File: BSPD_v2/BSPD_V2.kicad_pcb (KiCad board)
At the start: 2 copper layers, 85.5 x 52 mm, 0 parts

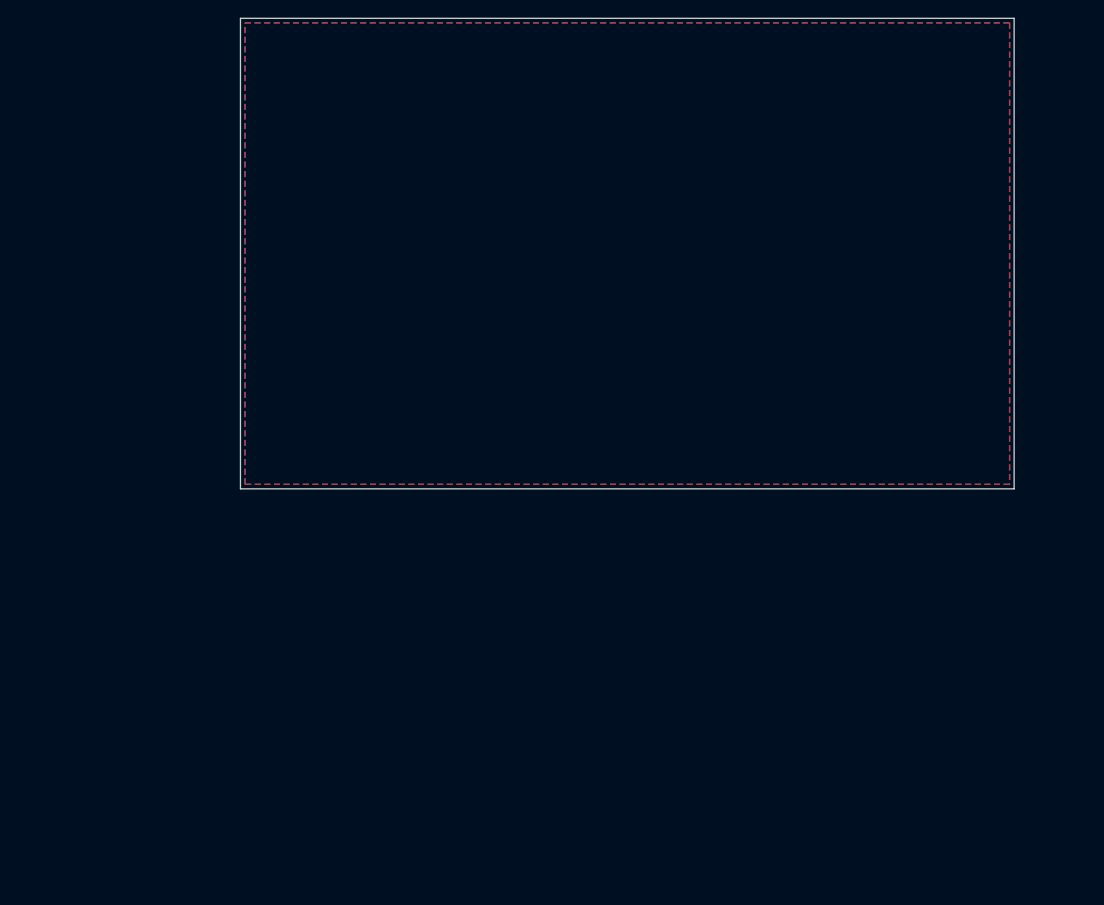
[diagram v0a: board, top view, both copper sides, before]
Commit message: Updated pcb design
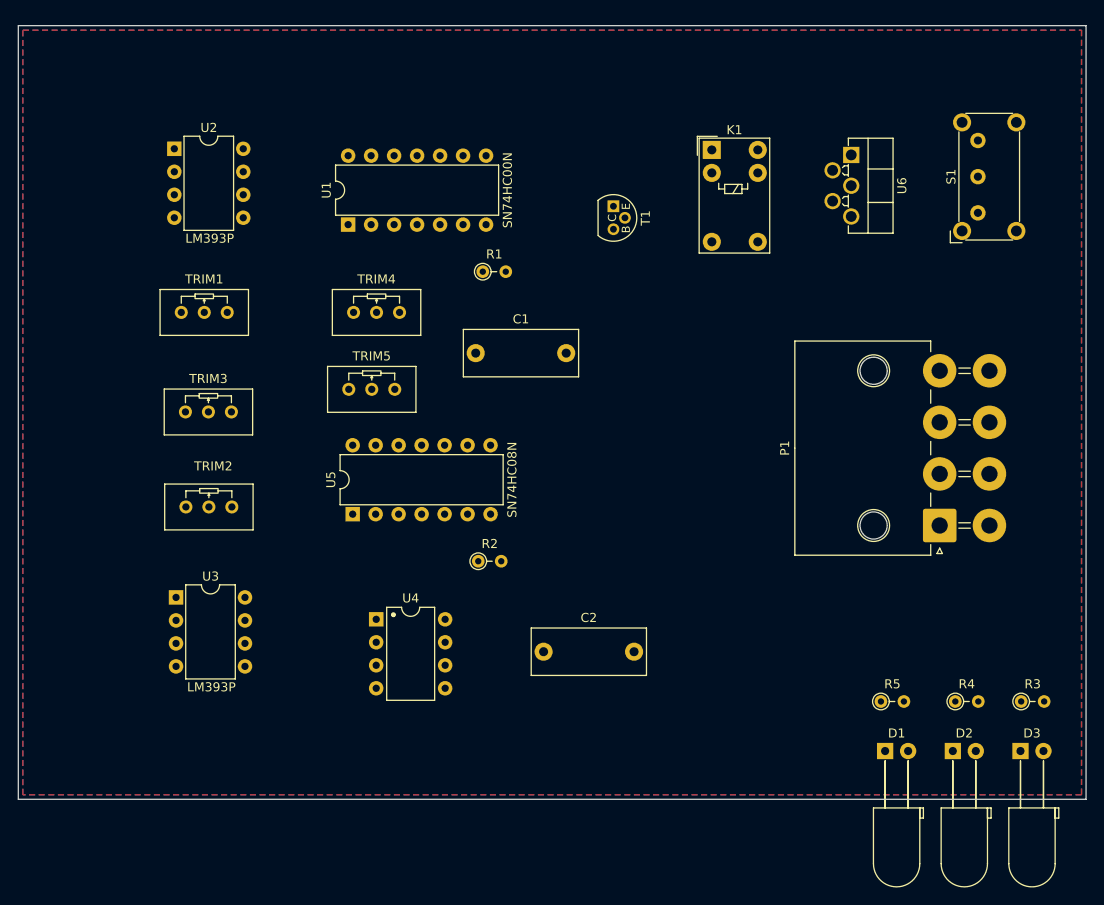
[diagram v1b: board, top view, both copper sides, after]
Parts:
- added C1: C_Generic, Capacitor_THT:C_Disc_D12.5mm_W5.0mm_P10.00mm, F.Cu at (107.5, 86.5)
- added C2: C_Generic, Capacitor_THT:C_Disc_D12.5mm_W5.0mm_P10.00mm, F.Cu at (115.0, 119.5)
- added D1: LED, LED_THT:LED_D5.0mm_Horizontal_O6.35mm_Z9.0mm, F.Cu at (152.7, 130.5)
- added D2: LED, LED_THT:LED_D5.0mm_Horizontal_O6.35mm_Z9.0mm, F.Cu at (160.2, 130.5)
- added D3: LED, LED_THT:LED_D5.0mm_Horizontal_O6.35mm_Z9.0mm, F.Cu at (167.7, 130.5)
- added K1: G5V-1, Relay_THT:Relay_SPDT_Omron_G5V-1, F.Cu at (133.6, 64.0)
- added P1: 0430450827, Connector_Molex:Molex_Mega-Fit_76825-0008_2x04_P5.70mm_Horizontal, F.Cu at (158.8, 105.5)
- added R1: R, PCM_Resistor_THT_AKL:R_Axial_DIN0204_L3.6mm_D1.6mm_P2.54mm_Vertical, F.Cu at (108.3, 77.5)
- added R2: R, PCM_Resistor_THT_AKL:R_Axial_DIN0204_L3.6mm_D1.6mm_P2.54mm_Vertical, F.Cu at (107.8, 109.5)
- added R3: R, PCM_Resistor_THT_AKL:R_Axial_DIN0204_L3.6mm_D1.6mm_P2.54mm_Vertical, F.Cu at (167.8, 125.0)
- added R4: R, PCM_Resistor_THT_AKL:R_Axial_DIN0204_L3.6mm_D1.6mm_P2.54mm_Vertical, F.Cu at (160.5, 125.0)
- added R5: R, PCM_Resistor_THT_AKL:R_Axial_DIN0204_L3.6mm_D1.6mm_P2.54mm_Vertical, F.Cu at (152.3, 125.0)
- added S1: EG1206, Button_Switch_THT:SW_E-Switch_EG1224_SPDT_Angled, F.Cu at (163.0, 71.0)
- added T1: T-BJT-NPN, PCM_Package_TO_SOT_THT_AKL_OneLayer:TO-92L_ECB, F.Cu at (122.7, 70.3)
- added TRIM1: TrimPot_TC33X_1k, PCM_Potentiometer_THT_AKL_Double:Potentiometer_Bourns_3296W_Vertical, F.Cu at (80.0, 82.0)
- added TRIM2: TrimPot_T73YEt_1k, PCM_Potentiometer_THT_AKL_Double:Potentiometer_Bourns_3296W_Vertical, F.Cu at (80.5, 103.5)
- added TRIM3: TrimPot_T73YEt_1k, PCM_Potentiometer_THT_AKL_Double:Potentiometer_Bourns_3296W_Vertical, F.Cu at (80.5, 93.0)
- added TRIM4: TrimPot_T73YEt_10k, PCM_Potentiometer_THT_AKL_Double:Potentiometer_Bourns_3296W_Vertical, F.Cu at (99.1, 82.0)
- added TRIM5: TrimPot_T73YEt_10k, PCM_Potentiometer_THT_AKL_Double:Potentiometer_Bourns_3296W_Vertical, F.Cu at (98.5, 90.5)
- added U1: SN74HC00N, PCM_4ms_Package_DIP:DIP-14_W7.62mm, F.Cu at (93.5, 72.3)
- added U2: LM393P, PCM_4ms_Package_DIP:DIP-8pin_TH, F.Cu at (74.2, 63.9)
- added U3: LM393P, PCM_4ms_Package_DIP:DIP-8pin_TH, F.Cu at (74.4, 113.5)
- added U4: LM393P, PCM_Package_DIP_AKL:DIP-8_W7.62mm, F.Cu at (96.5, 115.9)
- added U5: SN74HC08N, PCM_4ms_Package_DIP:DIP-14_W7.62mm, F.Cu at (94.0, 104.3)
- added U6: LM2596T-5, PCM_Package_TO_SOT_THT_AKL:TO-220F-5_P3.4x2.06mm_StaggerEven_Lead1.86mm_Vertical, F.Cu at (149.0, 64.6)
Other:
- board size 85.5 x 52 mm -> 118 x 85.5 mm
